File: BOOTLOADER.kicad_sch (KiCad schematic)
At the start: 17 parts, among them J4 Conn_01x02, J5 Conn_01x02, Q3 PMBT2222A, U3 TS5A3159DBVR, U4 W25Q128JVS

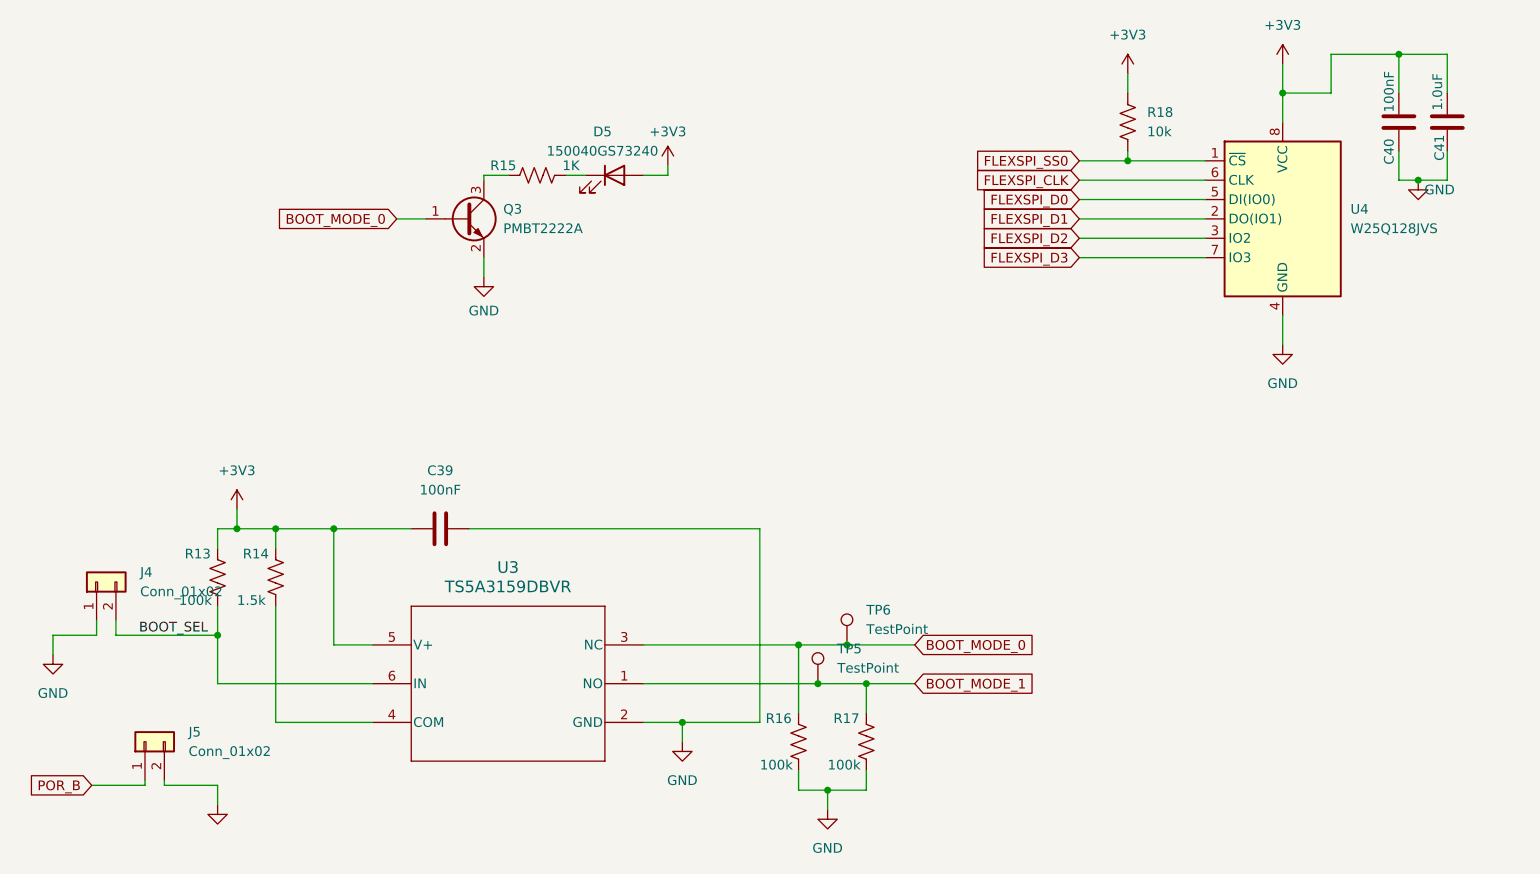
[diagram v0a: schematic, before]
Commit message: dad
da
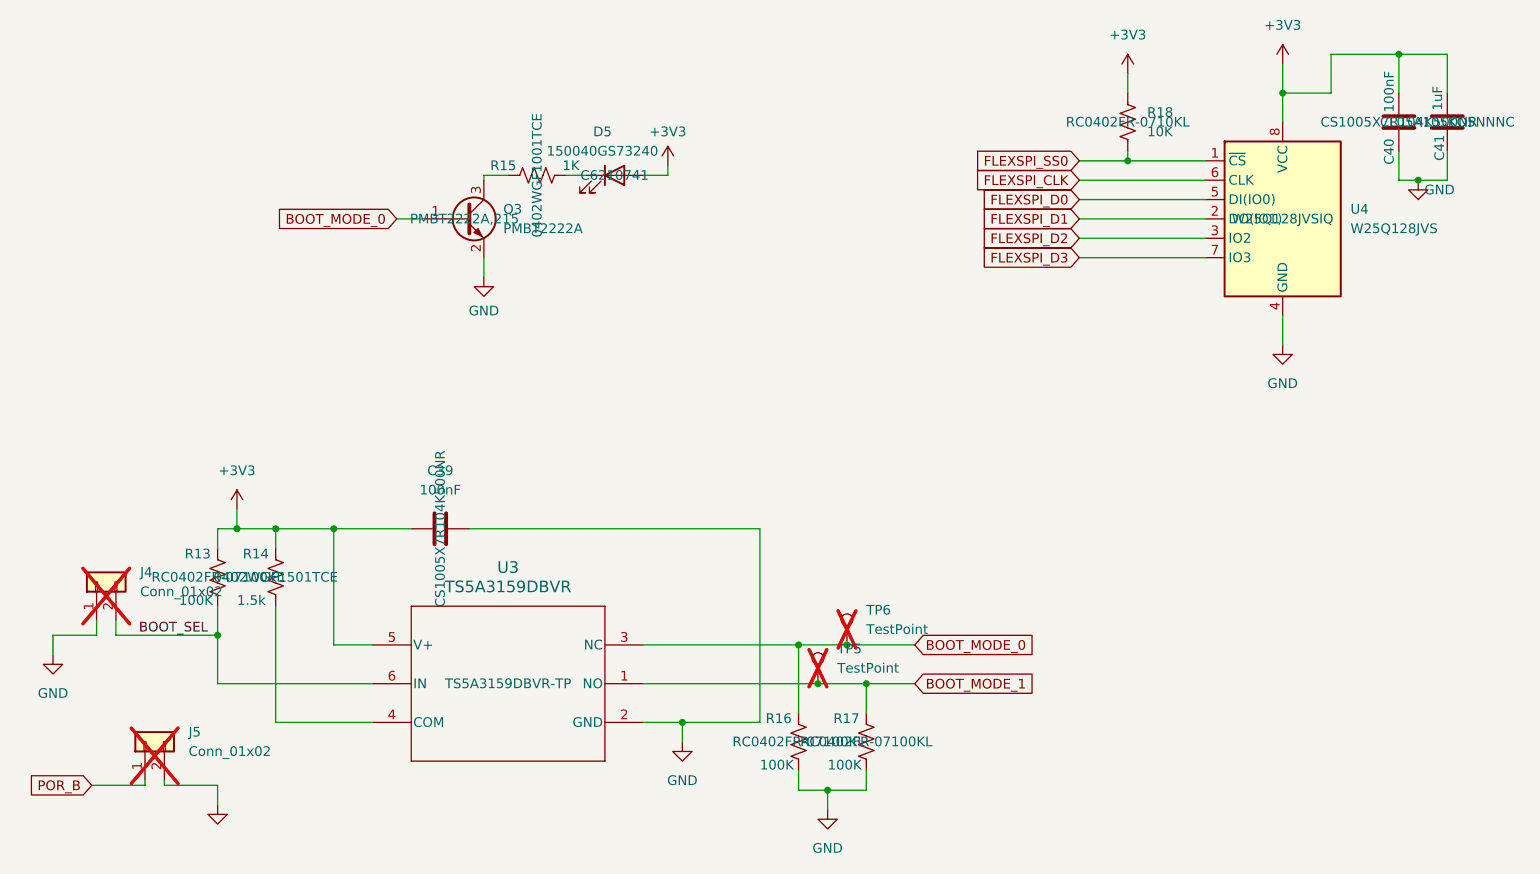
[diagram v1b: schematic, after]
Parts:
- C39, C40: Manufacturer_Part_Number (none) -> CS1005X7R104K500NR
- C41: value 1.0uF -> 1uF; Manufacturer_Part_Number (none) -> CL05A105KO5NNNC
- D5: Manufacturer_Part_Number (none) -> C6210741
- J4, J5, TP5, TP6: now not fitted
- Q3: Manufacturer_Part_Number (none) -> PMBT2222A,215
- R13, R16, R17: value 100k -> 100K; Manufacturer_Part_Number (none) -> RC0402FR-07100KL
- R14: Manufacturer_Part_Number (none) -> 0402WGF1501TCE
- R15: Manufacturer_Part_Number (none) -> 0402WGF1001TCE
- R18: value 10k -> 10K; Manufacturer_Part_Number (none) -> RC0402FR-0710KL
- U3: Manufacturer_Part_Number (none) -> TS5A3159DBVR-TP
- U4: Manufacturer_Part_Number (none) -> W25Q128JVSIQ
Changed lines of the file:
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@@
 			)
 		)
-		(property "Manufacturer_Part_Number" ""
+		(property "Manufacturer_Part_Number" "PMBT2222A,215"
 			(at 73.025 49.53 0)
 			(effects
@@
 			)
 		)
+		(property "partNum" ""
+			(at 73.025 49.53 0)
+			(effects
+				(font
+					(size 1.27 1.27)
+				)
+			)
+		)
 		(pin "3"
 		)
@@
 			)
 		)
-		(property "Value" "1.0uF"
+		(property "Value" "1uF"
 			(at 200.66 35.306 90)
 			(effects
@@
 			)
 		)
-		(property "Manufacturer_Part_Number" ""
+		(property "Manufacturer_Part_Number" "CL05A105KO5NNNC"
 			(at 201.93 36.83 0)
 			(effects
@@
 			)
 		)
+		(property "partNum" ""
+			(at 201.93 36.83 0)
+			(effects
+				(font
+					(size 1.27 1.27)
+				)
+			)
+		)
 		(pin "1"
 		)
@@
 			)
 		)
-		(property "Manufacturer_Part_Number" ""
+		(property "Manufacturer_Part_Number" "C6210741"
 			(at 92.71 43.815 0)
 			(effects
@@
 			)
 		)
+		(property "partNum" ""
+			(at 92.71 43.815 0)
+			(effects
+				(font
+					(size 1.27 1.27)
+				)
+			)
+		)
 		(pin "1"
 		)
@@
 			)
 		)
-		(property "Manufacturer_Part_Number" ""
+		(property "Manufacturer_Part_Number" "TS5A3159DBVR-TP"
 			(at 78.74 110.49 0)
 			(effects
@@
 			)
 		)
+		(property "partNum" ""
+			(at 78.74 110.49 0)
+			(effects
+				(font
+					(size 1.27 1.27)
+				)
+			)
+		)
 		(pin "2"
 		)
@@
 			)
 		)
-		(property "Manufacturer_Part_Number" ""
+		(property "Manufacturer_Part_Number" "CS1005X7R104K500NR"
 			(at 69.85 90.17 0)
 			(effects
@@
 			)
 		)
+		(property "partNum" ""
+			(at 69.85 90.17 0)
+			(effects
+				(font
+					(size 1.27 1.27)
+				)
+			)
+		)
 		(pin "2"
 		)
@@
 		(in_bom yes)
 		(on_board yes)
-		(dnp no)
+		(dnp yes)
 		(fields_autoplaced yes)
 		(property "Reference" "J5"
@@
 			)
 		)
+		(property "partNum" ""
+			(at 31.115 118.11 0)
+			(effects
+				(font
+					(size 1.27 1.27)
+				)
+			)
+		)
 		(pin "1"
 		)
@@
 			)
 		)
-		(property "Value" "10k"
+		(property "Value" "10K"
 			(at 162.56 38.0999 0)
 			(effects
@@
 			)
 		)
-		(property "Manufacturer_Part_Number" ""
+		(property "Manufacturer_Part_Number" "RC0402FR-0710KL"
 			(at 160.02 36.83 0)
 			(effects
@@
 			)
 		)
+		(property "partNum" ""
+			(at 160.02 36.83 0)
+			(effects
+				(font
+					(size 1.27 1.27)
+				)
+			)
+		)
 		(pin "1"
 		)
@@
 			)
 		)
-		(property "Manufacturer_Part_Number" ""
+		(property "Manufacturer_Part_Number" "0402WGF1001TCE"
 			(at 82.55 43.815 0)
 			(effects
@@
 			)
 		)
+		(property "partNum" ""
+			(at 82.55 43.815 0)
+			(effects
+				(font
+					(size 1.27 1.27)
+				)
+			)
+		)
 		(pin "1"
 		)
@@
 			)
 		)
-		(property "Value" "100k"
+		(property "Value" "100K"
 			(at 111.76 121.158 0)
 			(effects
@@
 			)
 		)
-		(property "Manufacturer_Part_Number" ""
+		(property "Manufacturer_Part_Number" "RC0402FR-07100KL"
 			(at 116.84 118.11 0)
 			(effects
@@
 			)
 		)
+		(property "partNum" ""
+			(at 116.84 118.11 0)
+			(effects
+				(font
+					(size 1.27 1.27)
+				)
+			)
+		)
 		(pin "2"
 		)
@@
 			)
 		)
-		(property "Value" "100k"
+		(property "Value" "100K"
 			(at 35.56 99.568 0)
 			(effects
@@
 			)
 		)
-		(property "Manufacturer_Part_Number" ""
+		(property "Manufacturer_Part_Number" "RC0402FR-07100KL"
 			(at 40.64 96.52 0)
 			(effects
@@
 			)
 		)
+		(property "partNum" ""
+			(at 40.64 96.52 0)
+			(effects
+				(font
+					(size 1.27 1.27)
+				)
+			)
+		)
 		(pin "2"
 		)
@@
 		(in_bom yes)
 		(on_board yes)
-		(dnp no)
+		(dnp yes)
 		(fields_autoplaced yes)
 		(property "Reference" "TP6"
@@
 			)
 		)
+		(property "partNum" ""
+			(at 123.19 105.41 0)
+			(effects
+				(font
+					(size 1.27 1.27)
+				)
+			)
+		)
 		(pin "1"
 		)
@@
 			)
 		)
-		(property "Manufacturer_Part_Number" ""
+		(property "Manufacturer_Part_Number" "0402WGF1501TCE"
 			(at 48.26 96.52 0)
 			(effects
@@
 			)
 		)
+		(property "partNum" ""
+			(at 48.26 96.52 0)
+			(effects
+				(font
+					(size 1.27 1.27)
+				)
+			)
+		)
 		(pin "2"
 		)
@@
 		(in_bom yes)
 		(on_board yes)
-		(dnp no)
+		(dnp yes)
 		(fields_autoplaced yes)
 		(property "Reference" "TP5"
@@
 			)
 		)
+		(property "partNum" ""
+			(at 119.38 110.49 0)
+			(effects
+				(font
+					(size 1.27 1.27)
+				)
+			)
+		)
 		(pin "1"
 		)
@@
 			)
 		)
-		(property "Value" "100k"
+		(property "Value" "100K"
 			(at 120.65 121.158 0)
 			(effects
@@
 			)
 		)
-		(property "Manufacturer_Part_Number" ""
+		(property "Manufacturer_Part_Number" "RC0402FR-07100KL"
 			(at 125.73 118.11 0)
 			(effects
@@
 			)
 		)
+		(property "partNum" ""
+			(at 125.73 118.11 0)
+			(effects
+				(font
+					(size 1.27 1.27)
+				)
+			)
+		)
 		(pin "2"
 		)
@@
 			)
 		)
-		(property "Manufacturer_Part_Number" ""
+		(property "Manufacturer_Part_Number" "W25Q128JVSIQ"
 			(at 180.34 49.53 0)
 			(effects
@@
 			)
 		)
+		(property "partNum" ""
+			(at 180.34 49.53 0)
+			(effects
+				(font
+					(size 1.27 1.27)
+				)
+			)
+		)
 		(pin "6"
 		)
@@
 			)
 		)
-		(property "Manufacturer_Part_Number" ""
+		(property "Manufacturer_Part_Number" "CS1005X7R104K500NR"
 			(at 195.58 36.83 0)
 			(effects
@@
 			)
 		)
+		(property "partNum" ""
+			(at 195.58 36.83 0)
+			(effects
+				(font
+					(size 1.27 1.27)
+				)
+			)
+		)
 		(pin "1"
 		)
@@
 		(in_bom yes)
 		(on_board yes)
-		(dnp no)
+		(dnp yes)
 		(fields_autoplaced yes)
 		(property "Reference" "J4"
@@
 			(at 24.765 97.155 0)
 			(effects
+				(font
+					(size 1.27 1.27)
+				)
+			)
+		)
+		(property "partNum" ""
+			(at 24.765 97.155 0)
+			(effects

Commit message: gema
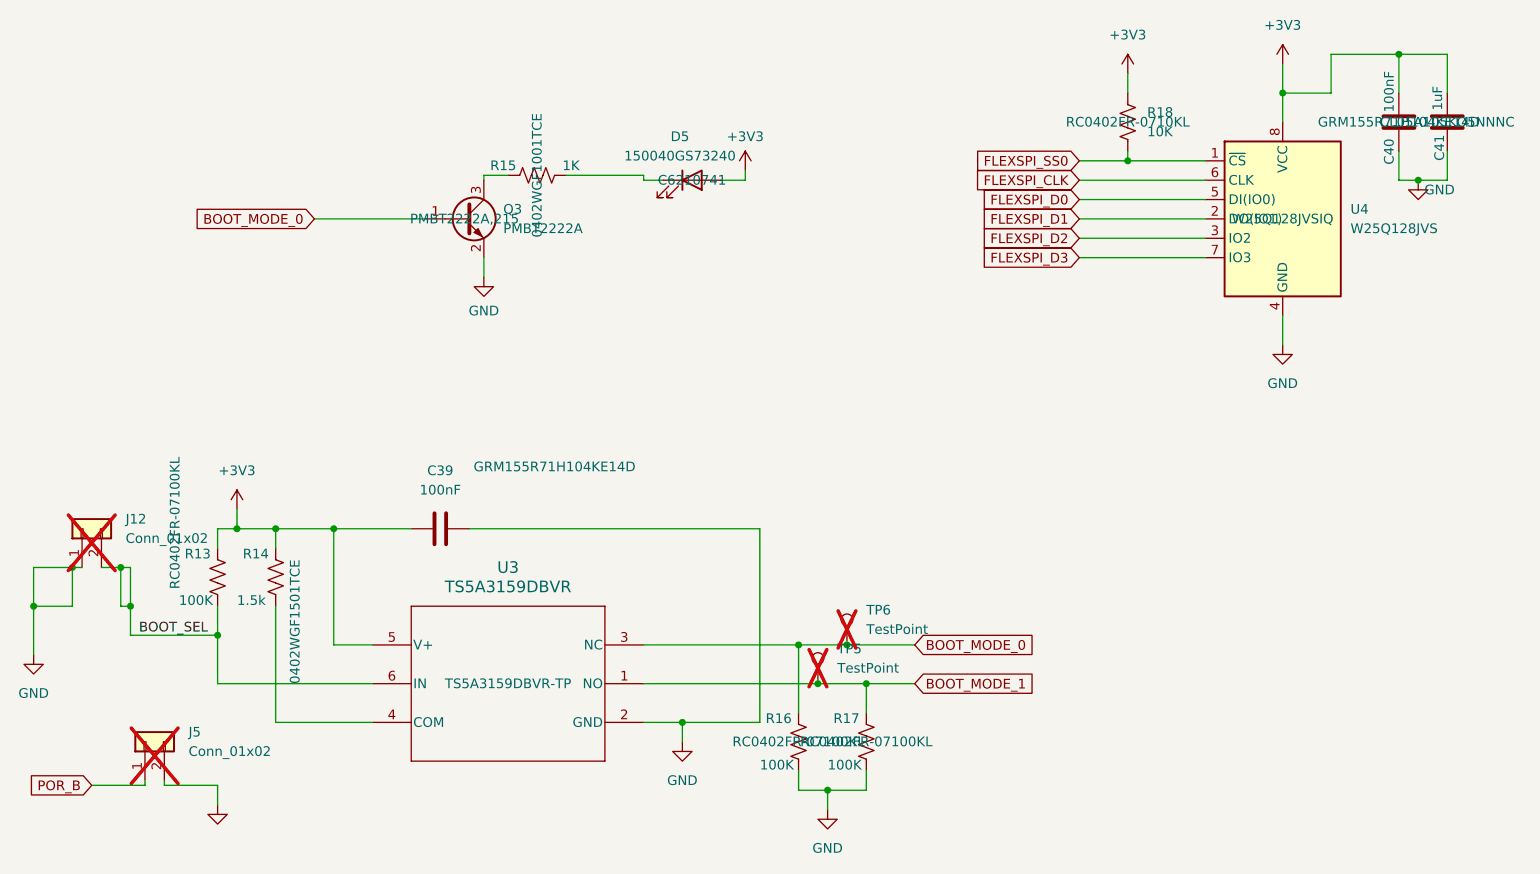
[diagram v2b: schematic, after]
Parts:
- removed J4: Conn_01x02, Connector_PinHeader_2.54mm:PinHeader_1x02_P2.54mm_Vertical, symbol Connector_Generic:Conn_01x02
- added J12: Conn_01x02, Connector_PinHeader_2.54mm:PinHeader_1x02_P2.54mm_Vertical, symbol Connector_Generic:Conn_01x02
- C39, C40:  LCSC Part # (none) -> C77020; Manufacturer_Part_Number CS1005X7R104K500NR -> GRM155R71H104KE14D
- C41:  LCSC Part # (none) -> C29266
- D5:  LCSC Part # (none) -> C6210741
- Q3:  LCSC Part # (none) -> C23869
- R13, R16, R17:  LCSC Part # (none) -> C60491
- R14:  LCSC Part # (none) -> C25867
- R15:  LCSC Part # (none) -> C11702
- R18:  LCSC Part # (none) -> C60490
- U3:  LCSC Part # (none) -> C42411032
- U4:  LCSC Part # (none) -> C97521
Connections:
- net BOOT_SEL: now also J12.2 (Pin_2)
- net GND: now also J12.1 (Pin_1)
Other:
- moved on the sheet: D5
